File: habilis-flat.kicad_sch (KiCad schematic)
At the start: 73 parts, among them J1 AudioJack4, SW1 MX, SW10 MX, SW11 MX, SW12 MX, SW13 MX, SW14 MX, SW15 MX, SW16 MX, SW17 MX, SW18 MX, SW19 MX, SW2 MX, SW20 MX, SW21 MX, SW22 MX, SW23 MX, SW24 MX, SW25 MX, SW26 MX, SW27 MX, SW28 MX, SW29 MX, SW3 MX, SW31 MX, SW32 MX, SW33 MX, SW34 MX, SW35 MX, SW36 MX, SW4 MX, SW5 MX, SW6 MX, SW7 MX, SW8 MX, SW9 MX, U1 ProMicro

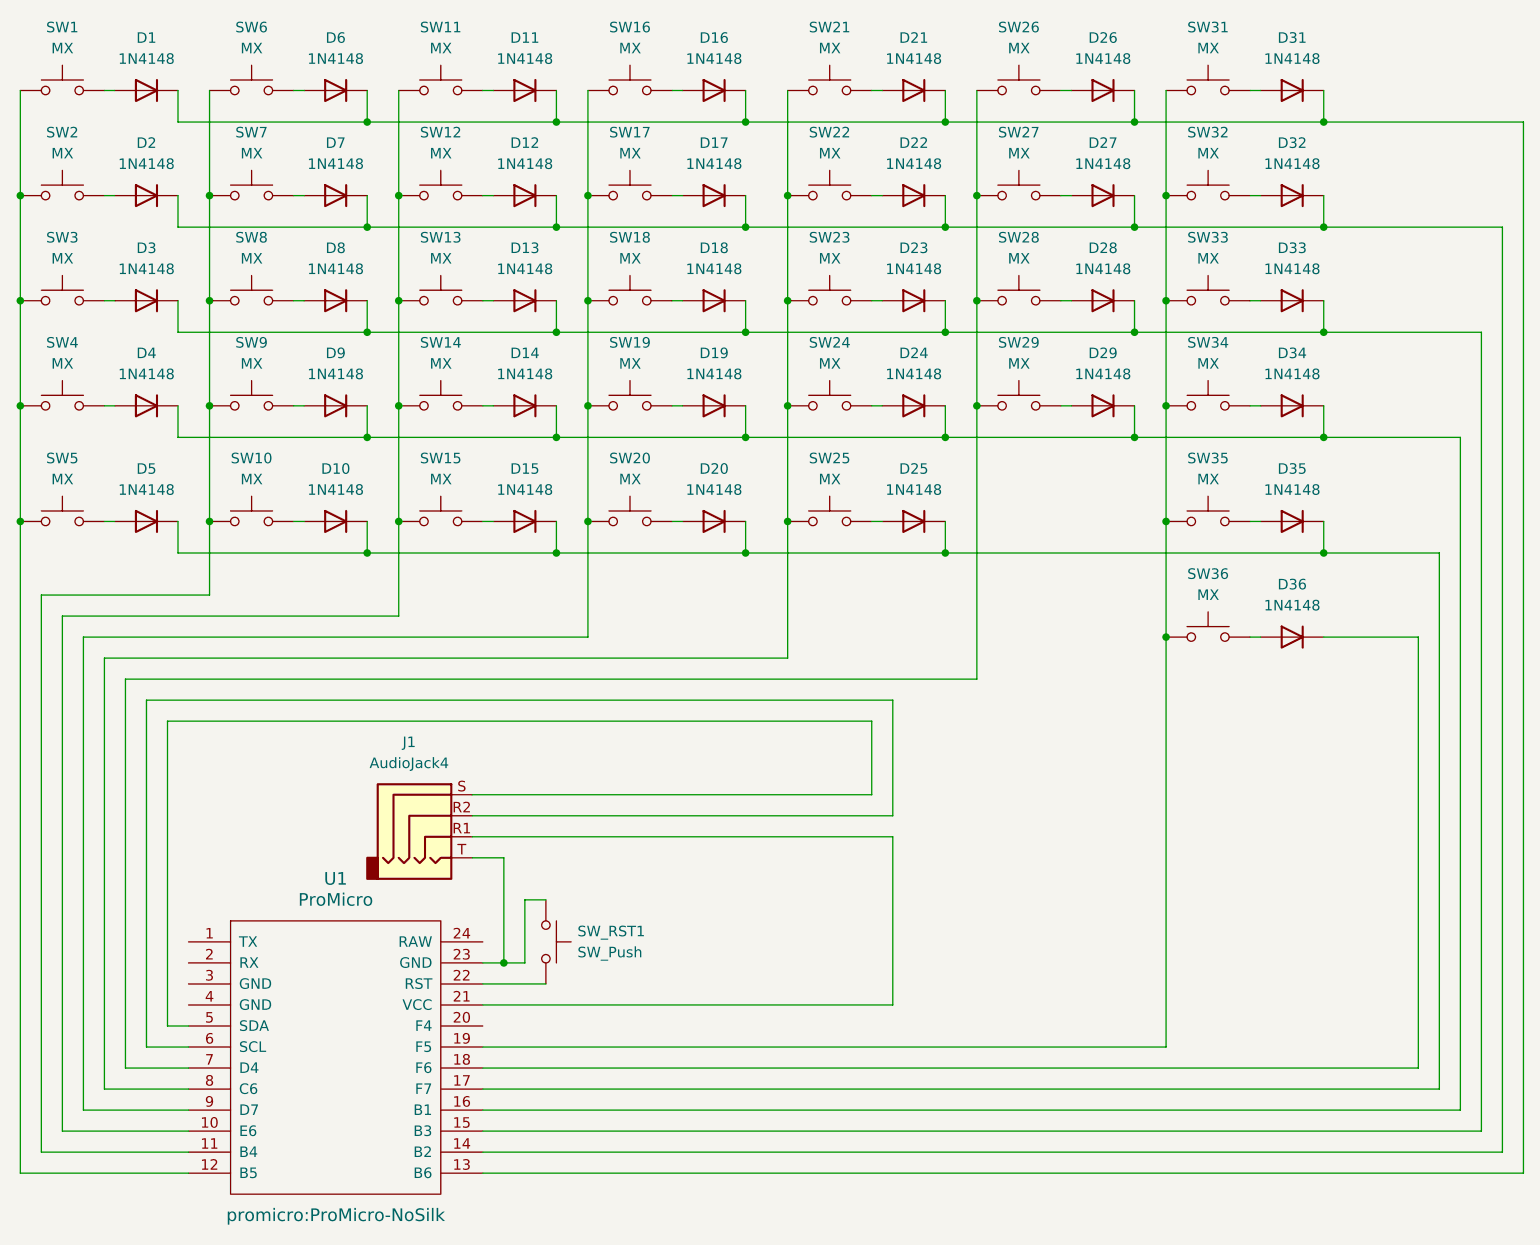
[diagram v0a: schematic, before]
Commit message: Revision 1
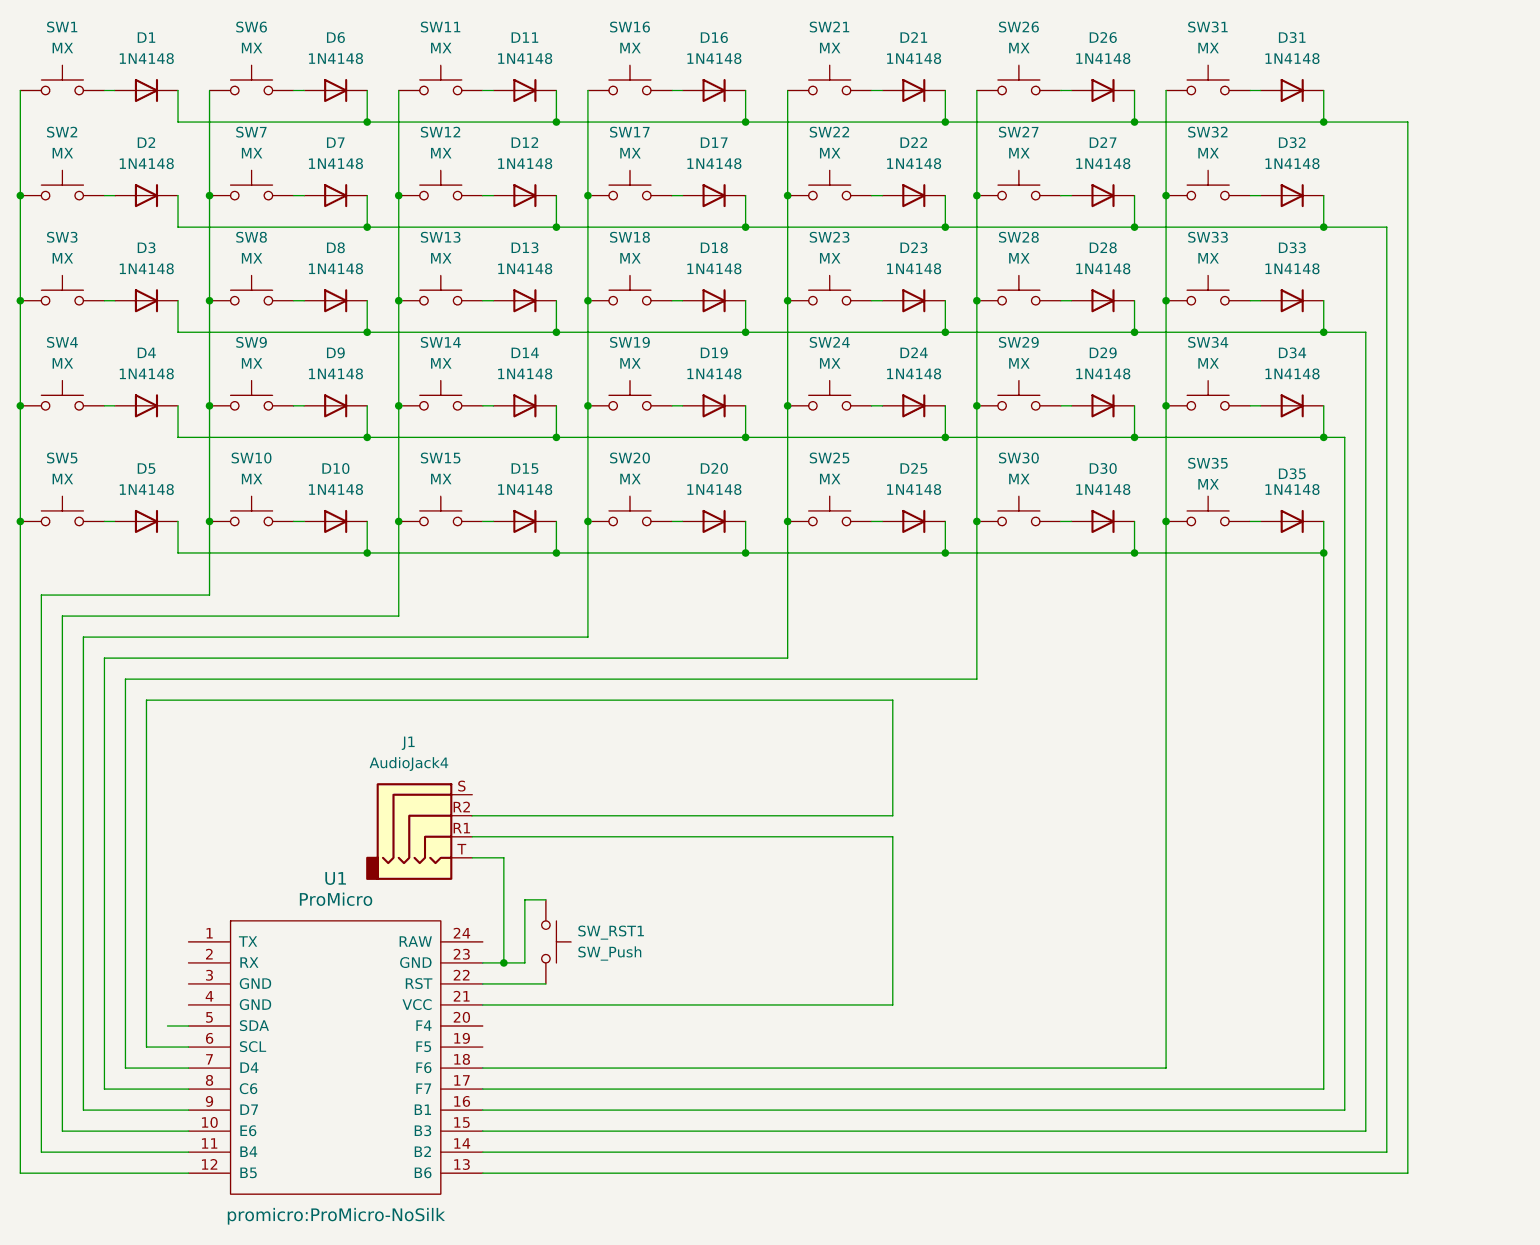
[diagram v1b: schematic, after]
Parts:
- removed D36: 1N4148, Diode_THT:D_DO-35_SOD27_P7.62mm_Horizontal, symbol Diode:1N4148
- added D35: 1N4148, Diode_THT:D_DO-35_SOD27_P7.62mm_Horizontal, symbol Diode:1N4148
- renumbered D31 to D30, D32 to D31, D33 to D32, D34 to D33, D35 to D34, SW31 to SW30, SW32 to SW31, SW33 to SW32, SW34 to SW33, SW35 to SW34, SW36 to SW35
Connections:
- net at D14.1 (K), D19.1 (K), D24.1 (K)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: now also D34.1 (K); no longer D33.1 (K)
- net at D10.1 (K), D15.1 (K), D20.1 (K)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: now also D30.1 (K), D35.1 (K); no longer D34.1 (K)
- net at SW26.2, SW27.2, SW28.2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: now also SW30.2
- net at D1.1 (K), D11.1 (K), D16.1 (K)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: now also D31.1 (K); no longer D30.1 (K)
- net at J1.S: no longer U1.5 (SDA)
- net at SW31.2, SW32.2, SW34.2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: now also SW33.1, U1.18 (F6); no longer SW30.2, SW33.2, U1.19 (F5)
- net at D12.1 (K), D17.1 (K), D2.1 (K)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: now also D32.1 (K); no longer D31.1 (K)
- net at SW35.1: now also D35.2 (A)
- net at D13.1 (K), D18.1 (K), D23.1 (K)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: now also D33.1 (K); no longer D32.1 (K)
- net at D33.2 (A): now also SW33.2; no longer SW33.1
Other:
- moved on the sheet: D30, D31, D32, D33, D34, SW30, SW31, SW32, SW33, SW34, SW35

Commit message: Revision 2
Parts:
- J1: footprint Connector_PinHeader_2.54mm:PinHeader_1x04_P2.54mm_Vertical -> project-components:Jack breakout board
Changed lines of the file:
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@@
       (effects (font (size 1.27 1.27)))
     )
-    (property "Footprint" "Connector_PinHeader_2.54mm:PinHeader_1x04_P2.54mm_Vertical" (at 85.09 120.65 0)
+    (property "Footprint" "project-components:Jack breakout board" (at 85.09 120.65 0)
       (effects (font (size 1.27 1.27)) hide)
     )
